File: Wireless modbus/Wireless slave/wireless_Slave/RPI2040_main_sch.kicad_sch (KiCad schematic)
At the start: 6 parts, among them J3 Conn_01x02, U1 RP2040, U2 W25Q128JVS, Y1 Crystal

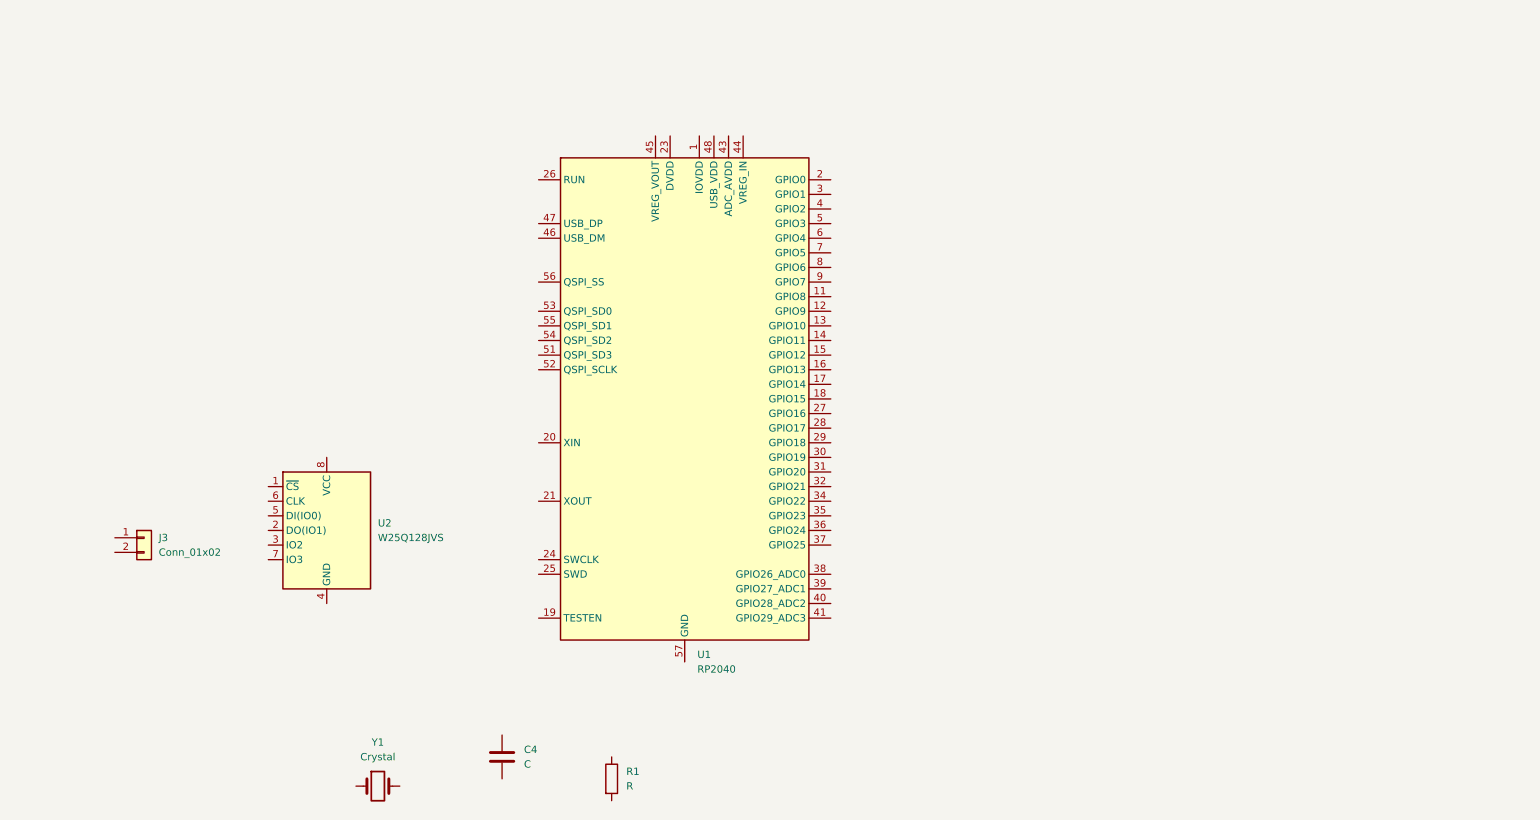
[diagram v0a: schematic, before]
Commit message: ændringer
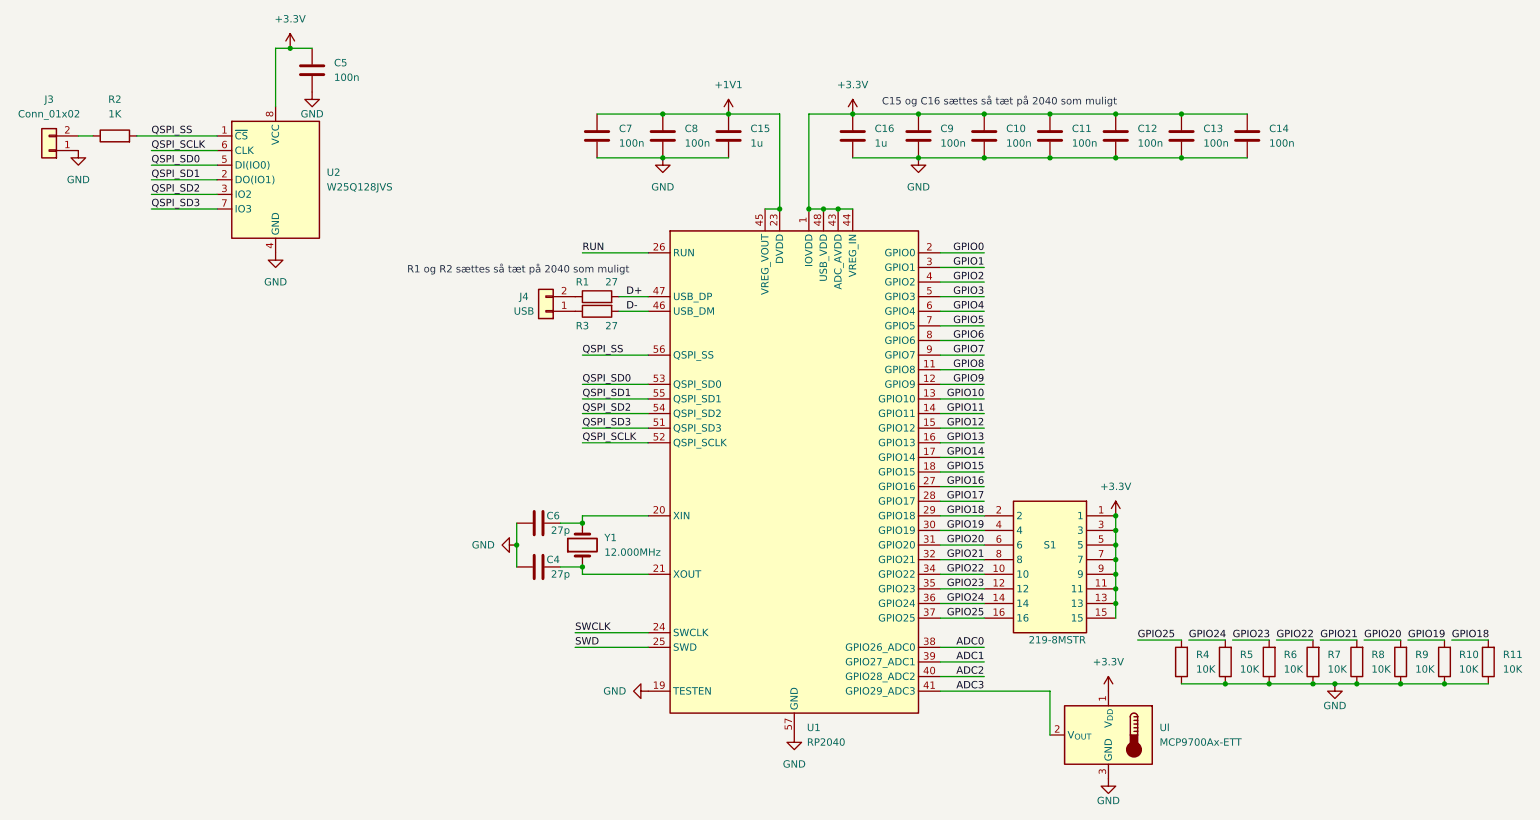
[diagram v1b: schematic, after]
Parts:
- added C10, C11, C12, C13, C14, C5, C7, C8, C9: 100n, symbol Device:C
- added C15, C16: 1u, symbol Device:C
- added C6: 27p, symbol Device:C
- added J4: USB, symbol Connector_Generic:Conn_01x02
- added R10, R11, R4, R5, R6, R7, R8, R9: 10K, symbol Device:R
- added R2: 1K, symbol Device:R
- added R3: 27, symbol Device:R
- added S1: 219-8MSTR, 2198MSTR, symbol SamacSys_Parts:219-8MSTR
- added Ul: MCP9700Ax-ETT, Package_TO_SOT_SMD:SOT-23, symbol Sensor_Temperature:MCP9700Ax-ETT
- C4: value C -> 27p
- R1: value R -> 27
- U1: JLCPCB (none) -> C2040
- U2: JLCPCB (none) -> C97521
- Y1: value Crystal -> 12.000MHz
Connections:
- net at R1.1: now also J4.2 (Pin_2)
- net D+: now reaches R1.2
- net D+: now also U1.47 (USB_DP)
- net at Y1.1: now also C4.2, U1.21 (XOUT)
- net at Y1.2: now also U1.20 (XIN), C6.2
- net GND: now reaches J3.1 (Pin_1)
- net GND: now also C4.1, U1.19 (TESTEN), U1.57 (GND), U2.4 (GND), C10.2, C11.2, C12.2, C13.2, C14.2, C15.2, C16.2, C5.2, C6.1, C7.2, C8.2, C9.2, R10.1, R11.1, R4.1, R5.1, R6.1, R7.1, R8.1, R9.1, Ul.3 (GND)
- net at J3.2 (Pin_2): now also R2.1
- net QSPI_SS: now reaches U2.1 (~{CS})
- net QSPI_SS: now also U1.56 (QSPI_SS), R2.2
- net QSPI_SD1: now reaches U2.2 (DO(IO1))
- net QSPI_SD1: now also U1.55 (QSPI_SD1)
- net QSPI_SD2: now reaches U2.3 (IO2)
- net QSPI_SD2: now also U1.54 (QSPI_SD2)
- net QSPI_SD0: now reaches U2.5 (DI(IO0))
- net QSPI_SD0: now also U1.53 (QSPI_SD0)
- net QSPI_SCLK: now reaches U2.6 (CLK)
- net QSPI_SCLK: now also U1.52 (QSPI_SCLK)
- net QSPI_SD3: now reaches U2.7 (IO3)
- net QSPI_SD3: now also U1.51 (QSPI_SD3)
- net +3.3V: now reaches U2.8 (VCC)
- net +3.3V: now also U1.1 (IOVDD), U1.10 (IOVDD), U1.22 (IOVDD), U1.33 (IOVDD), U1.42 (IOVDD), U1.43 (ADC_AVDD), U1.44 (VREG_IN), U1.48 (USB_VDD), U1.49 (IOVDD), C10.1, C11.1, C12.1, C13.1, C14.1, C16.1, C5.1, C9.1, S1.1, S1.11, S1.13, S1.15, S1.3, S1.5, S1.7, S1.9, Ul.1 (V_{DD})
- net GPIO8: now reaches U1.11 (GPIO8)
- net GPIO9: now reaches U1.12 (GPIO9)
- net GPIO10: now reaches U1.13 (GPIO10)
- net GPIO11: now reaches U1.14 (GPIO11)
- net GPIO12: now reaches U1.15 (GPIO12)
- net GPIO13: now reaches U1.16 (GPIO13)
- net GPIO14: now reaches U1.17 (GPIO14)
- net GPIO15: now reaches U1.18 (GPIO15)
- net GPIO0: now reaches U1.2 (GPIO0)
- net +1V1: now reaches U1.23 (DVDD), U1.50 (DVDD)
- net +1V1: now also U1.45 (VREG_VOUT), C15.1, C7.1, C8.1
- net SWCLK: now reaches U1.24 (SWCLK)
- net SWD: now reaches U1.25 (SWD)
- net RUN: now reaches U1.26 (RUN)
- net GPIO16: now reaches U1.27 (GPIO16)
- net GPIO17: now reaches U1.28 (GPIO17)
- net GPIO18: now reaches U1.29 (GPIO18)
- net GPIO18: now also R11.2, S1.2
- net GPIO1: now reaches U1.3 (GPIO1)
- net GPIO19: now reaches U1.30 (GPIO19)
- net GPIO19: now also R10.2, S1.4
- net GPIO20: now reaches U1.31 (GPIO20)
- net GPIO20: now also R9.2, S1.6
- net GPIO21: now reaches U1.32 (GPIO21)
- net GPIO21: now also R8.2, S1.8
- net GPIO22: now reaches U1.34 (GPIO22)
- net GPIO22: now also R7.2, S1.10
- net GPIO23: now reaches U1.35 (GPIO23)
- net GPIO23: now also R6.2, S1.12
- net GPIO24: now reaches U1.36 (GPIO24)
- net GPIO24: now also R5.2, S1.14
- net GPIO25: now reaches U1.37 (GPIO25)
- net GPIO25: now also R4.2, S1.16
- net ADC0: now reaches U1.38 (GPIO26_ADC0)
- net ADC1: now reaches U1.39 (GPIO27_ADC1)
- net GPIO2: now reaches U1.4 (GPIO2)
- net ADC2: now reaches U1.40 (GPIO28_ADC2)
- net ADC3: now reaches U1.41 (GPIO29_ADC3)
- net ADC3: now also Ul.2 (V_{OUT})
- net D-: now reaches U1.46 (USB_DM)
- net D-: now also R3.2
- net GPIO3: now reaches U1.5 (GPIO3)
- net GPIO4: now reaches U1.6 (GPIO4)
- net GPIO5: now reaches U1.7 (GPIO5)
- net GPIO6: now reaches U1.8 (GPIO6)
- net GPIO7: now reaches U1.9 (GPIO7)
- new net: J4.1 (Pin_1), R3.1
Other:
- note added: "C15 og C16 sættes så tæt på 2040 som muligt"
- note added: "R1 og R2 sættes så tæt på 2040 som muligt"
- moved on the sheet: C4, J3, U1, U2, Y1
